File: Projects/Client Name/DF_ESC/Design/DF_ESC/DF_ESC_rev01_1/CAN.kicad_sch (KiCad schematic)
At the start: 0 parts

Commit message: libraries & schemtics
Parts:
- added C40, C41: 51p, symbol Device:C
- added C42: 2u2, symbol Device:C
- added D6: ESDCAN24-2BLY, SOT95P255X125-3N, symbol ESDCAN24-2BLY:ESDCAN24-2BLY
- added FL1: 744227S, Inductor_THT:L_CommonMode_PulseElectronics_PH9455x105NL_1, symbol Filter:Choke_CommonMode_PulseElectronics_PH9455x105NL
- added J4: Conn_01x04, symbol Connector_Generic:Conn_01x04
- added R23: 120R, symbol Device:R
- added R24, R25: 10R, symbol Device:R
- added R26: 10K, symbol Device:R
- added U3: SN65HVD230, Package_SO:SOIC-8_3.9x4.9mm_P1.27mm, symbol Interface_CAN_LIN:SN65HVD230
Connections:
- new net: R26.1, U3.8 (Rs)
- new net: C40.2, R23.1, R25.1
- new net: C41.1, R23.2, R24.1
- new net +3V3: C42.1, U3.3 (VCC)
- new net +5V: J4.4 (Pin_4)
- new net CAN_RX: U3.4 (R)
- new net CAN_TX: U3.1 (D)
- new net GND: C40.1, C41.2, C42.2, D6.3 (I/O_3), J4.1 (Pin_1), R26.2, U3.2 (GND)
- no-connect marks 0 -> 1
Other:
- note added: "03407610395"
- note added: "BYPASS PLACE AS CLOSE AS POSSIBLE TO IC"
- note added: "CAN"
- note added: "CAN_H AND CAN_L TO BE ROUTED AS DIFFERENTIAL PAIR"
- note added: "MODE SELECTION RESISTOR SLEWRATE OF -15 V/μs MORE INFO ON DATASHEET"
- note added: "Muhammad Moiz"
- note added: "moizrai765yt@gmail.com"
- company: (none) -> coVenture
- title: (none) -> CAN

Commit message: updated footprints
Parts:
- C40, C41, C42: footprint (none) -> Capacitor_SMD:C_0603_1608Metric
- D6: footprint SOT95P255X125-3N -> ESDCAN24-2BLY:SOT95P255X125-3N
- J4: footprint (none) -> Connector_PinHeader_1.00mm:PinHeader_1x04_P1.00mm_Vertical
- R23, R24, R25, R26: footprint (none) -> Resistor_SMD:R_0201_0603Metric
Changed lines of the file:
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@@
 			)
 		)
-		(property "Footprint" ""
+		(property "Footprint" "Resistor_SMD:R_0201_0603Metric"
 			(at 132.842 66.04 90)
 			(effects
@@
 			)
 		)
-		(property "Footprint" ""
+		(property "Footprint" "Resistor_SMD:R_0201_0603Metric"
 			(at 215.392 80.01 90)
 			(effects
@@
 			)
 		)
-		(property "Footprint" ""
+		(property "Footprint" "Capacitor_SMD:C_0603_1608Metric"
 			(at 147.0152 88.9 0)
 			(effects
@@
 			)
 		)
-		(property "Footprint" "SOT95P255X125-3N"
+		(property "Footprint" "ESDCAN24-2BLY:SOT95P255X125-3N"
 			(at 118.11 69.85 0)
 			(effects
@@
 			)
 		)
-		(property "Footprint" ""
+		(property "Footprint" "Resistor_SMD:R_0201_0603Metric"
 			(at 149.86 57.658 90)
 			(effects
@@
 			)
 		)
-		(property "Footprint" ""
+		(property "Footprint" "Connector_PinHeader_1.00mm:PinHeader_1x04_P1.00mm_Vertical"
 			(at 74.93 67.31 0)
 			(effects
@@
 			)
 		)
-		(property "Footprint" ""
+		(property "Footprint" "Capacitor_SMD:C_0603_1608Metric"
 			(at 147.0152 50.8 0)
 			(effects
@@
 			)
 		)
-		(property "Footprint" ""
+		(property "Footprint" "Capacitor_SMD:C_0603_1608Metric"
 			(at 207.9752 49.53 0)
 			(effects
@@
 			)
 		)
-		(property "Footprint" ""
+		(property "Footprint" "Resistor_SMD:R_0201_0603Metric"
 			(at 149.86 77.978 90)
 			(effects

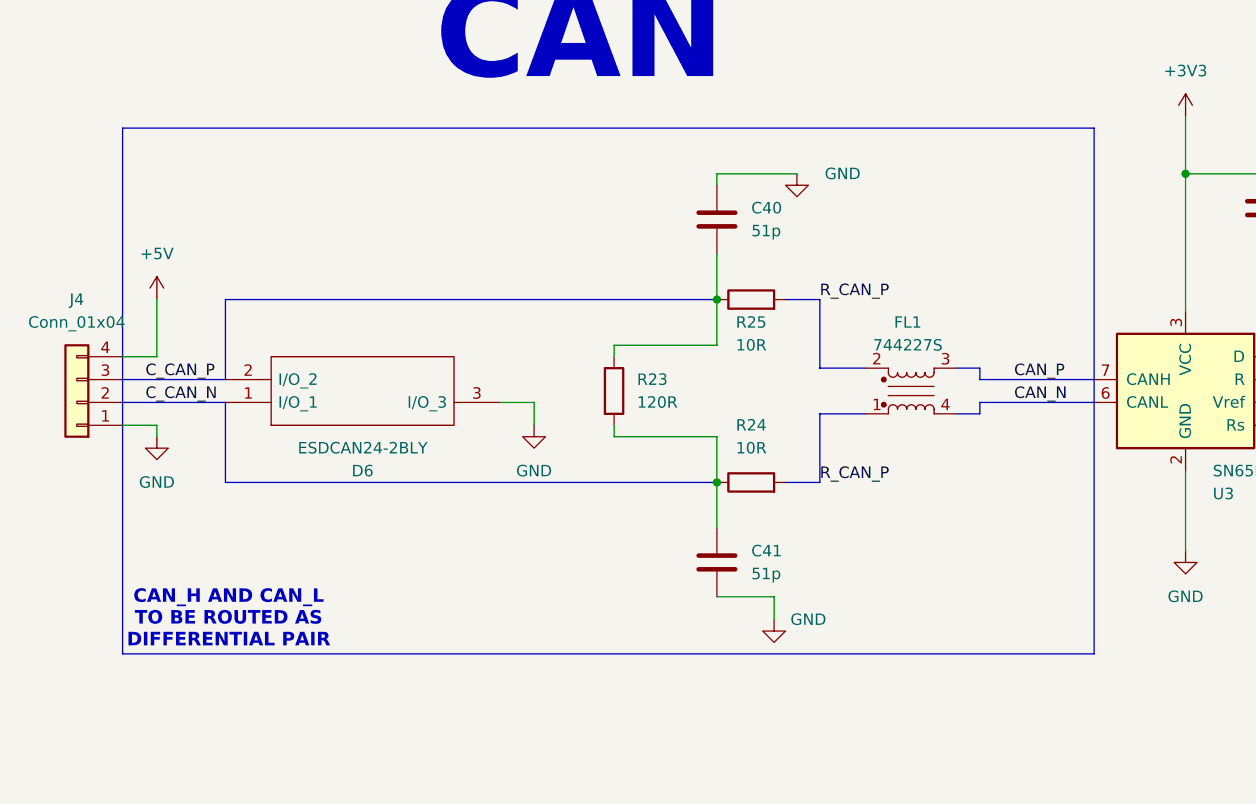
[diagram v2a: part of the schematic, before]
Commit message: UPDATED ERD ERRORS
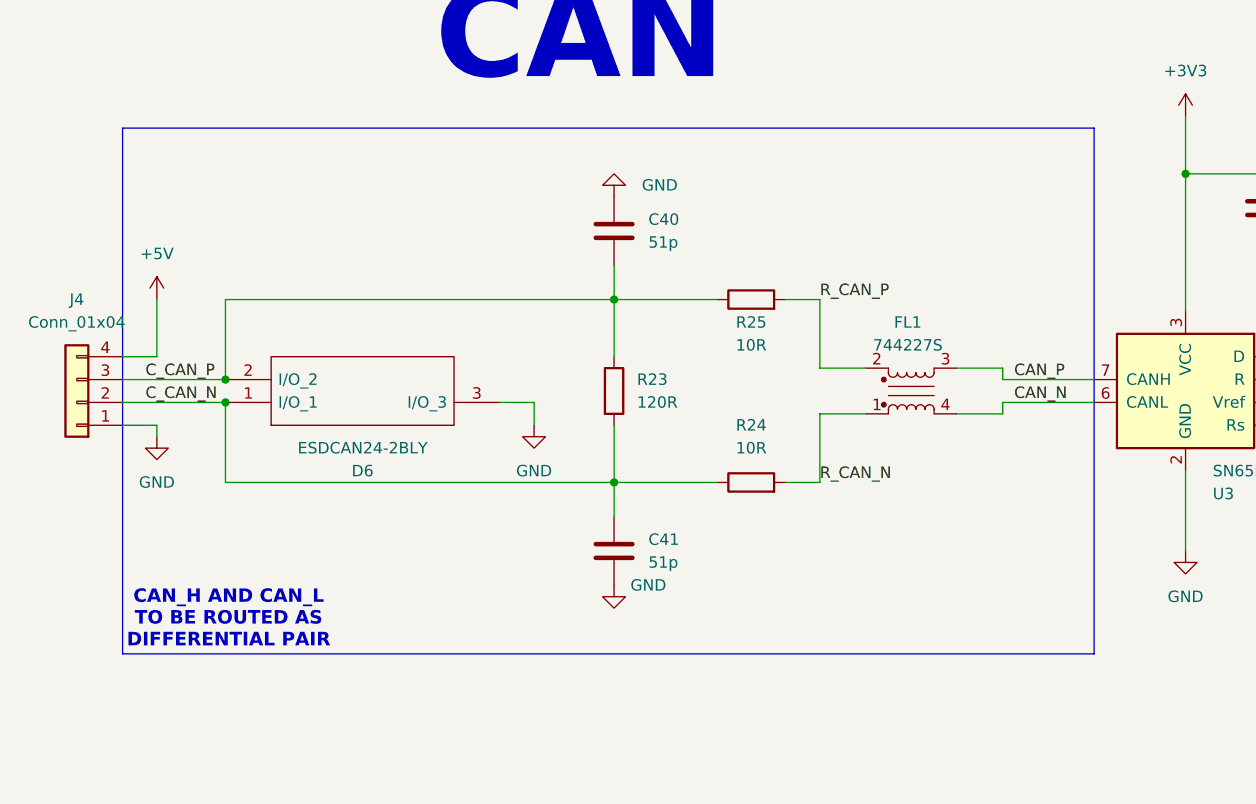
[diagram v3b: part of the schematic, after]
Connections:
- net CAN_N: now also FL1.4, U3.6 (CANL)
- net CAN_P: now also FL1.3, U3.7 (CANH)
- net C_CAN_N: now also C41.1, D6.1 (I/O_1), J4.2 (Pin_2), R23.2, R24.1
- net C_CAN_P: now also C40.2, D6.2 (I/O_2), J4.3 (Pin_3), R23.1, R25.1
- net R_CAN_P: now also FL1.2, R25.2
- net R_CAN_N: now reaches FL1.1
- net R_CAN_N: now also R24.2
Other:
- moved on the sheet: C40, C41
